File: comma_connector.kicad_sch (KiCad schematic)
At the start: 3 parts, among them J1 2317507-1, J3 Screw_Terminal_01x06, J4 Screw_Terminal_01x06

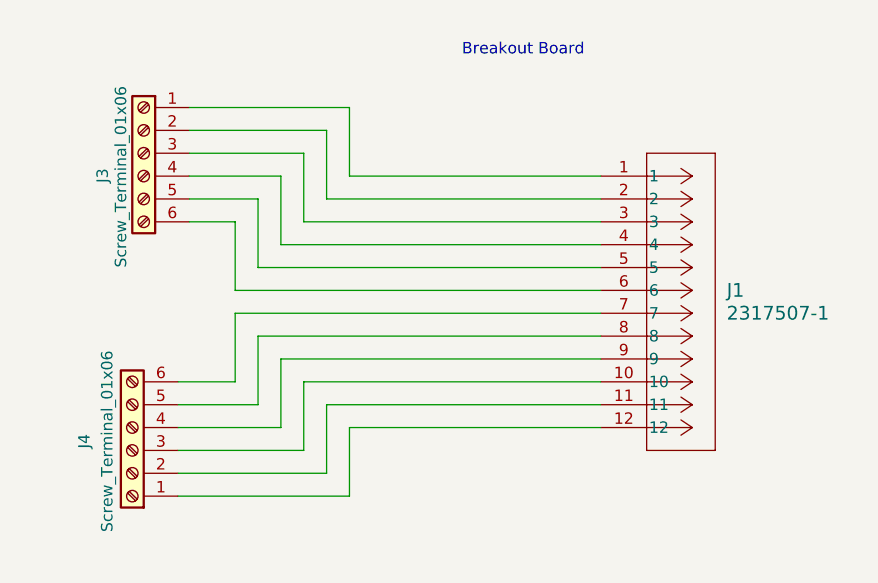
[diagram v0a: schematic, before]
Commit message: work in progress
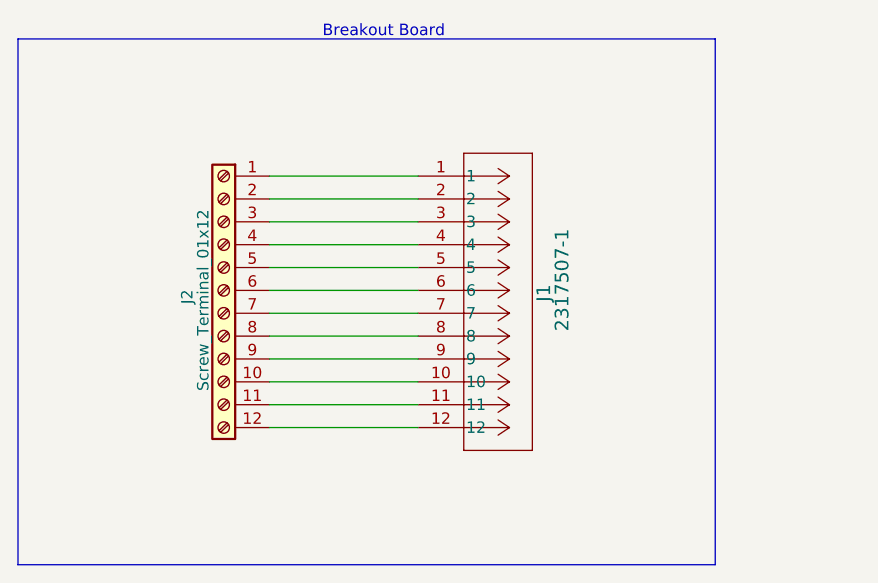
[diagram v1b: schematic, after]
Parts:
- removed J3, J4: Screw_Terminal_01x06, TerminalBlock:TerminalBlock_MaiXu_MX126-5.0-06P_1x06_P5.00mm, symbol Connector:Screw_Terminal_01x06
- added J2: Screw_Terminal_01x12, Connector_Phoenix_SPT:PhoenixContact_SPT_1.5_12-H-3.5_1x12_P3.5mm_Horizontal, symbol Connector:Screw_Terminal_01x12
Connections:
- net at J1.12: now also J2.12 (Pin_12)
- net at J1.11: now also J2.11 (Pin_11)
- net at J1.10: now also J2.10 (Pin_10)
- net at J1.9: now also J2.9 (Pin_9)
- net at J1.8: now also J2.8 (Pin_8)
- net at J1.7: now also J2.7 (Pin_7)
- net at J1.1: now also J2.1 (Pin_1)
- net at J1.2: now also J2.2 (Pin_2)
- net at J1.3: now also J2.3 (Pin_3)
- net at J1.4: now also J2.4 (Pin_4)
- net at J1.5: now also J2.5 (Pin_5)
- net at J1.6: now also J2.6 (Pin_6)
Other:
- moved on the sheet: J1

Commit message: update footprint to use 1x12 and 2.54mm pitch
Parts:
- J2: footprint Connector_Phoenix_SPT:PhoenixContact_SPT_1.5_12-H-3.5_1x12_P3.5mm_Horizontal -> TerminalBlock:TerminalBlock_MaiXu_MX126-5.0-12P_1x12_P5.00mm
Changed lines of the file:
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@@
 			)
 		)
-		(property "Footprint" "Connector_Phoenix_SPT:PhoenixContact_SPT_1.5_12-H-3.5_1x12_P3.5mm_Horizontal"
+		(property "Footprint" "TerminalBlock:TerminalBlock_MaiXu_MX126-5.0-12P_1x12_P5.00mm"
 			(at 105.41 115.57 0)
 			(hide yes)

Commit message: minor updates to PCB
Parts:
- J2: footprint TerminalBlock:TerminalBlock_MaiXu_MX126-5.0-12P_1x12_P5.00mm -> TerminalBlock:TerminalBlock_Xinya_XY308-2.54-12P_1x12_P2.54mm_Horizontal
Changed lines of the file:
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@@
 			)
 		)
-		(property "Footprint" "TerminalBlock:TerminalBlock_MaiXu_MX126-5.0-12P_1x12_P5.00mm"
+		(property "Footprint" "TerminalBlock:TerminalBlock_Xinya_XY308-2.54-12P_1x12_P2.54mm_Horizontal"
 			(at 105.41 115.57 0)
 			(hide yes)
